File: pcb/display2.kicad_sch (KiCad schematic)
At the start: 35 parts, among them Q13 2N7002K, Q14 2N7002K, Q15 2N7002K, Q16 2N7002K, Q17 BSS84, Q18 BSS84, Q19 BSS84, Q20 BSS84, Q21 BSS84, Q22 BSS84, Q23 BSS84, Q24 BSS84, U3 74HC595

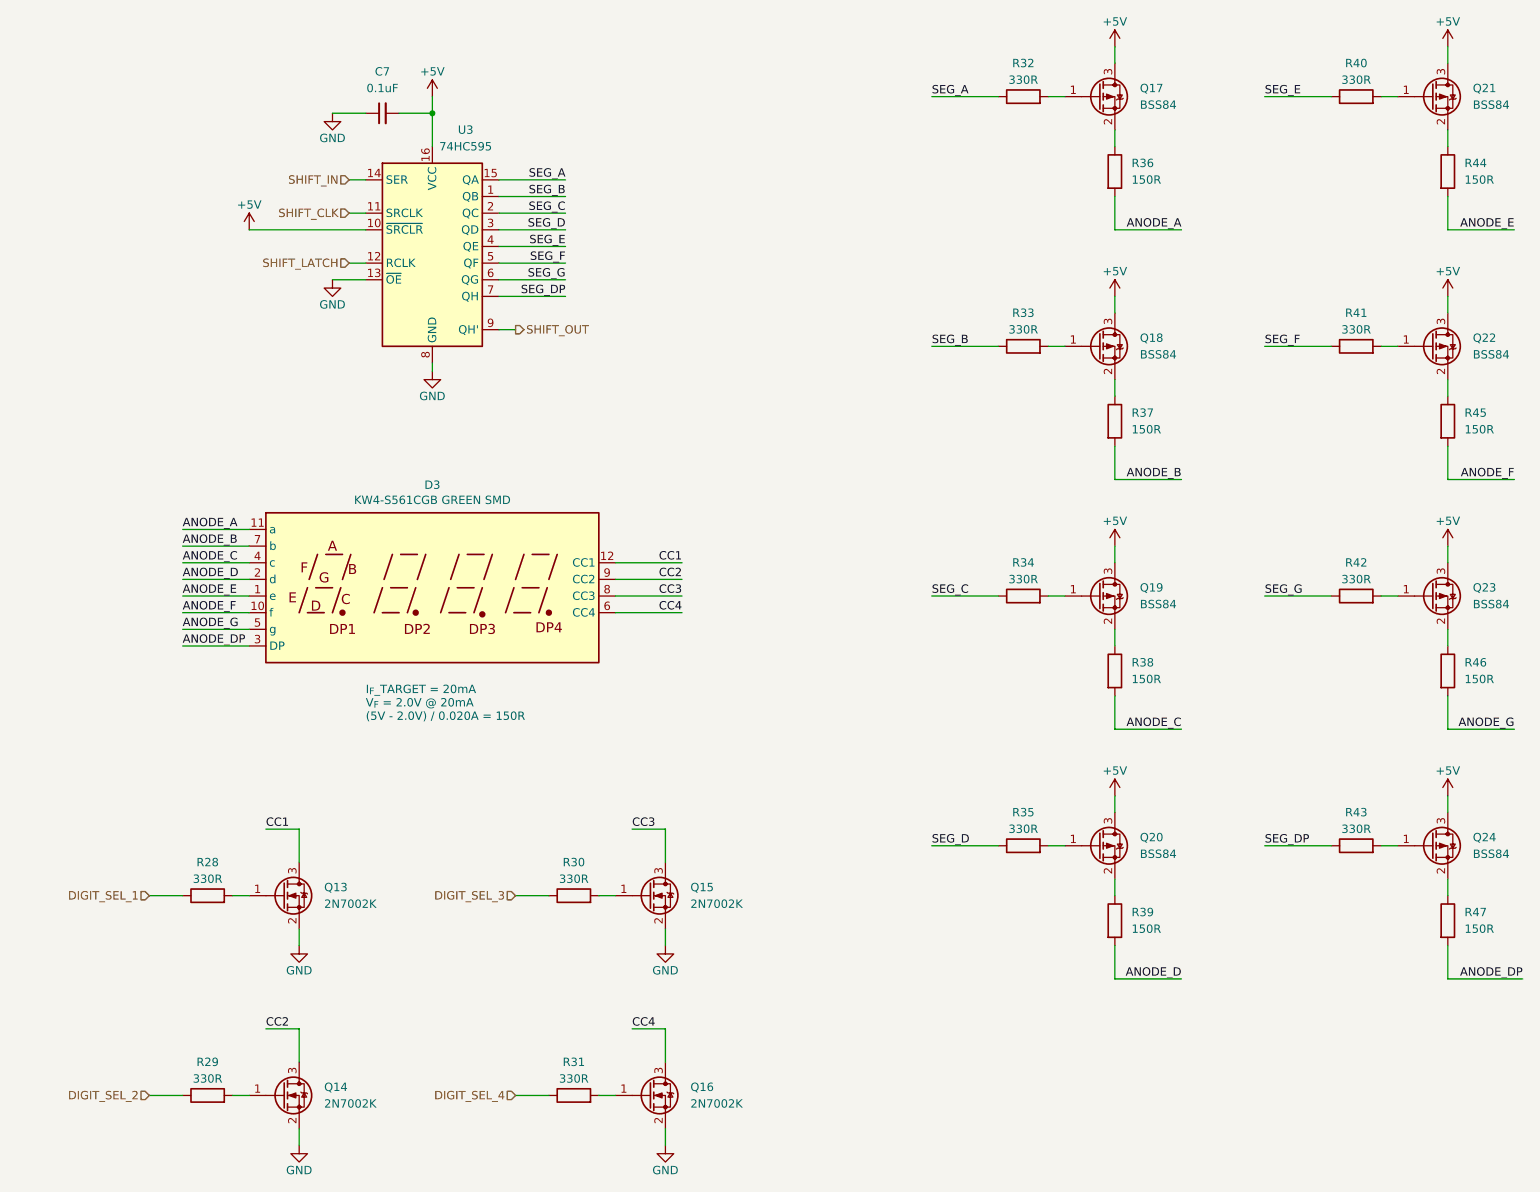
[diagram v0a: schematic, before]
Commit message: common anode schematic
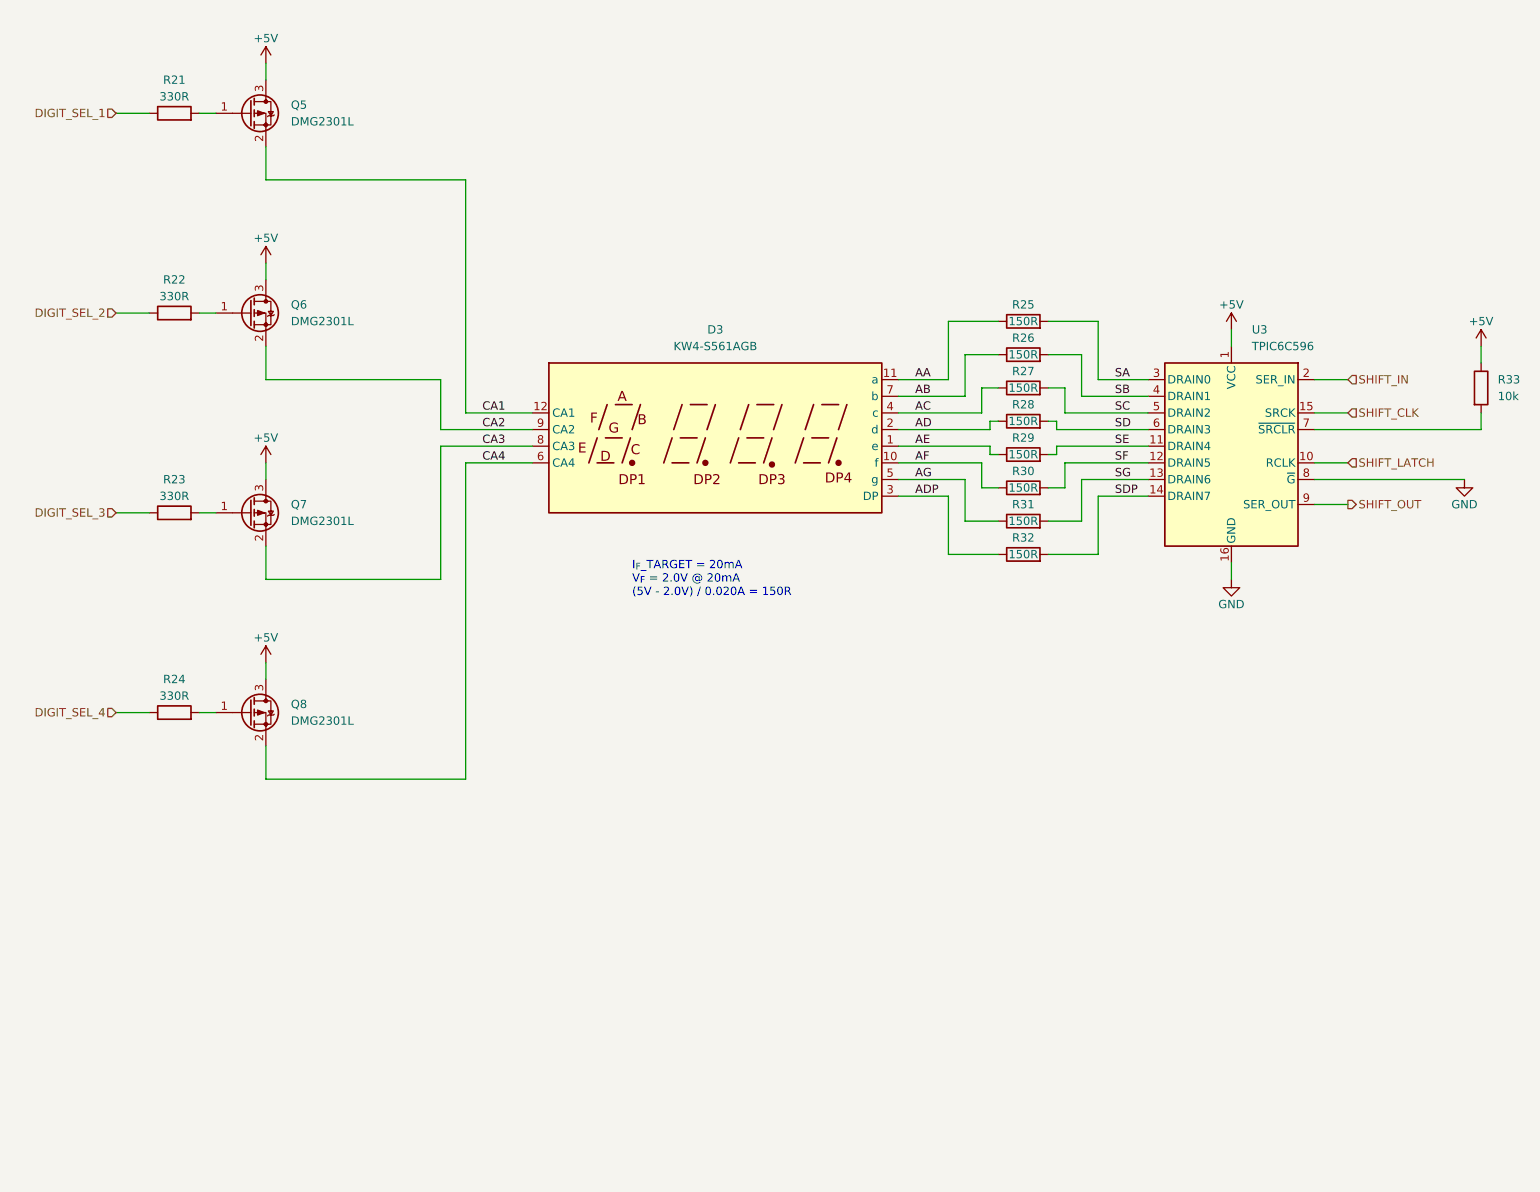
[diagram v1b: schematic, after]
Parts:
- removed C7: 0.1uF, Capacitor_SMD:C_0805_2012Metric_Pad1.18x1.45mm_HandSolder, symbol Device:C_Small
- removed D3: KW4-S561CGB GREEN SMD, mtg_life_counter:KW4-S561xxB_SMD, symbol mtg_life_counter:KW4-S561CxB
- removed Q13, Q14, Q15, Q16: 2N7002K, Package_TO_SOT_SMD:SOT-23, symbol Transistor_FET:2N7002K
- removed Q17, Q18, Q19, Q20, Q21, Q22, Q23, Q24: BSS84, Package_TO_SOT_SMD:SOT-23, symbol Transistor_FET:BSS84
- removed R34, R35, R40, R41, R42, R43: 330R, Resistor_SMD:R_0805_2012Metric_Pad1.20x1.40mm_HandSolder, symbol Device:R
- removed R36, R37, R38, R39, R44, R45, R46, R47: 150R, Resistor_SMD:R_0805_2012Metric_Pad1.20x1.40mm_HandSolder, symbol Device:R
- removed U3: 74HC595, Package_SO:SOIC-16_3.9x9.9mm_P1.27mm, symbol 74xx:74HC595
- added D3: KW4-S561AGB, mtg_life_counter:KW4-S561xxB_SMD, symbol mtg_life_counter:KW4-S561AxB
- added Q5, Q6, Q7, Q8: DMG2301L, Package_TO_SOT_SMD:SOT-23, symbol Transistor_FET:DMG2301L
- added R21, R22, R23, R24: 330R, Resistor_SMD:R_0805_2012Metric_Pad1.20x1.40mm_HandSolder, symbol Device:R
- added R25, R26, R27: 150R, Resistor_SMD:R_0805_2012Metric_Pad1.20x1.40mm_HandSolder, symbol Device:R
- added U3: TPIC6C596, Package_SO:SOIC-16_3.9x9.9mm_P1.27mm, symbol mtg_life_counter:TPIC6C596
- R28, R29, R30, R31, R32: value 330R -> 150R
- R33: value 330R -> 10k
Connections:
- net SEG_B is gone; now on net +5V: R33.1
- net +5V: now also Q5.3 (D), Q6.3 (D), Q7.3 (D), Q8.3 (D), U3.1 (VCC)
- net DIGIT_SEL_1: now also R21.1; no longer R28.1
- net DIGIT_SEL_2: now also R22.1; no longer R29.1
- net DIGIT_SEL_3: now also R23.1; no longer R30.1
- net DIGIT_SEL_4: now also R24.1; no longer R31.1
- net GND: now also U3.16 (GND), U3.8 (~{G})
- net SHIFT_CLK: now also U3.15 (SRCK)
- net SHIFT_IN: now also U3.2 (SER_IN)
- net SHIFT_LATCH: now also U3.10 (RCLK)
- net SHIFT_OUT: now also U3.9 (SER_OUT)
- net at R33.2: now also U3.7 (~{SRCLR})
- net SF: now reaches R30.2
- net SF: now also U3.12 (DRAIN5)
- net SE: now reaches R29.2
- net SE: now also U3.11 (DRAIN4)
- net SD: now reaches R28.2
- net SD: now also U3.6 (DRAIN3)
- net SG: now reaches R31.2
- net SG: now also U3.13 (DRAIN6)
- net SDP: now reaches R32.2
- net SDP: now also U3.14 (DRAIN7)
- net SEG_A renamed ADP
- net ADP: now also D3.3 (DP)
- new net: Q7.1 (G), R23.2
- new net: Q8.1 (G), R24.2
- new net: Q5.1 (G), R21.2
- new net: Q6.1 (G), R22.2
- new net AA: D3.11 (a), R25.1
- new net AB: D3.7 (b), R26.1
- new net AC: D3.4 (c), R27.1
- new net AD: D3.2 (d), R28.1
- new net AE: D3.1 (e), R29.1
- new net AF: D3.10 (f), R30.1
- new net AG: D3.5 (g), R31.1
- new net CA1: D3.12 (CA1), Q5.2 (S)
- new net CA2: D3.9 (CA2), Q6.2 (S)
- new net CA3: D3.8 (CA3), Q7.2 (S)
- new net CA4: D3.6 (CA4), Q8.2 (S)
- new net SA: R25.2, U3.3 (DRAIN0)
- new net SB: R26.2, U3.4 (DRAIN1)
- new net SC: R27.2, U3.5 (DRAIN2)
